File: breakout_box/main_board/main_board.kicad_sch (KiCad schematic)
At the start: 43 parts, among them CN1 19PIN_LEMO, Q1 DMP3099L, Q2 MJD122, Q3 AOZ1360AIL

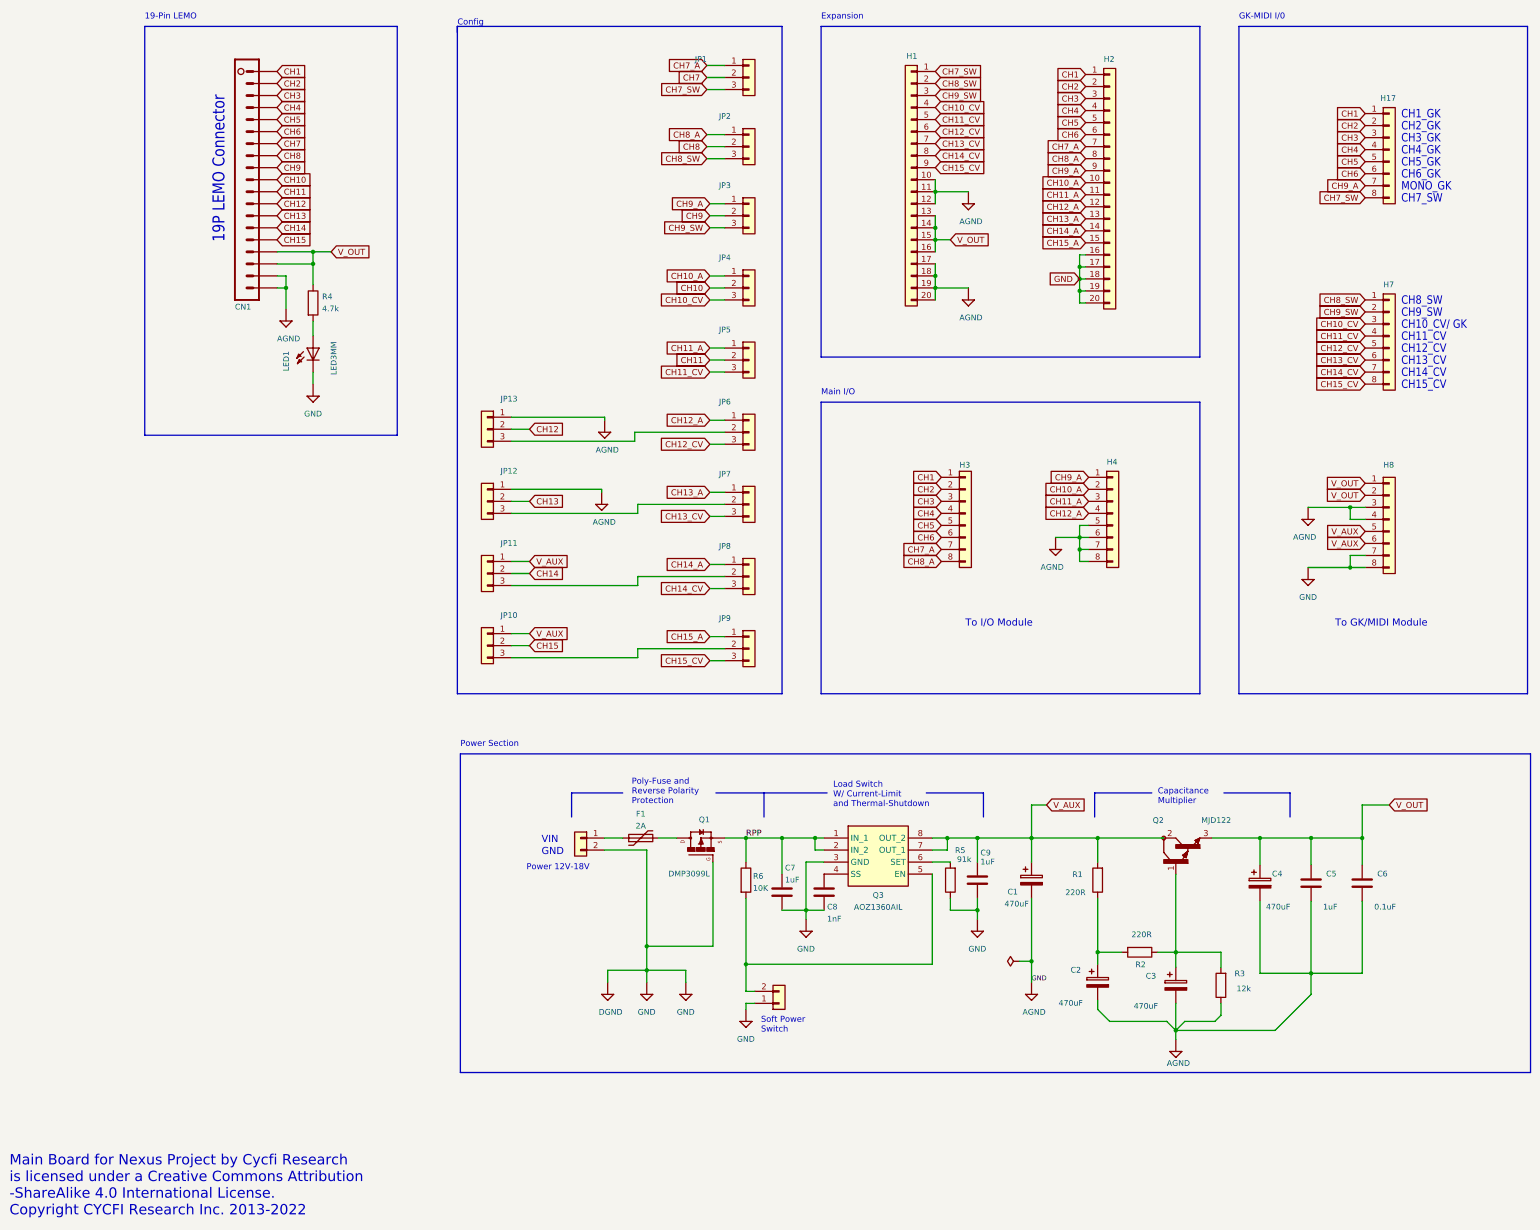
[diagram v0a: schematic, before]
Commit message: Production run May 2025
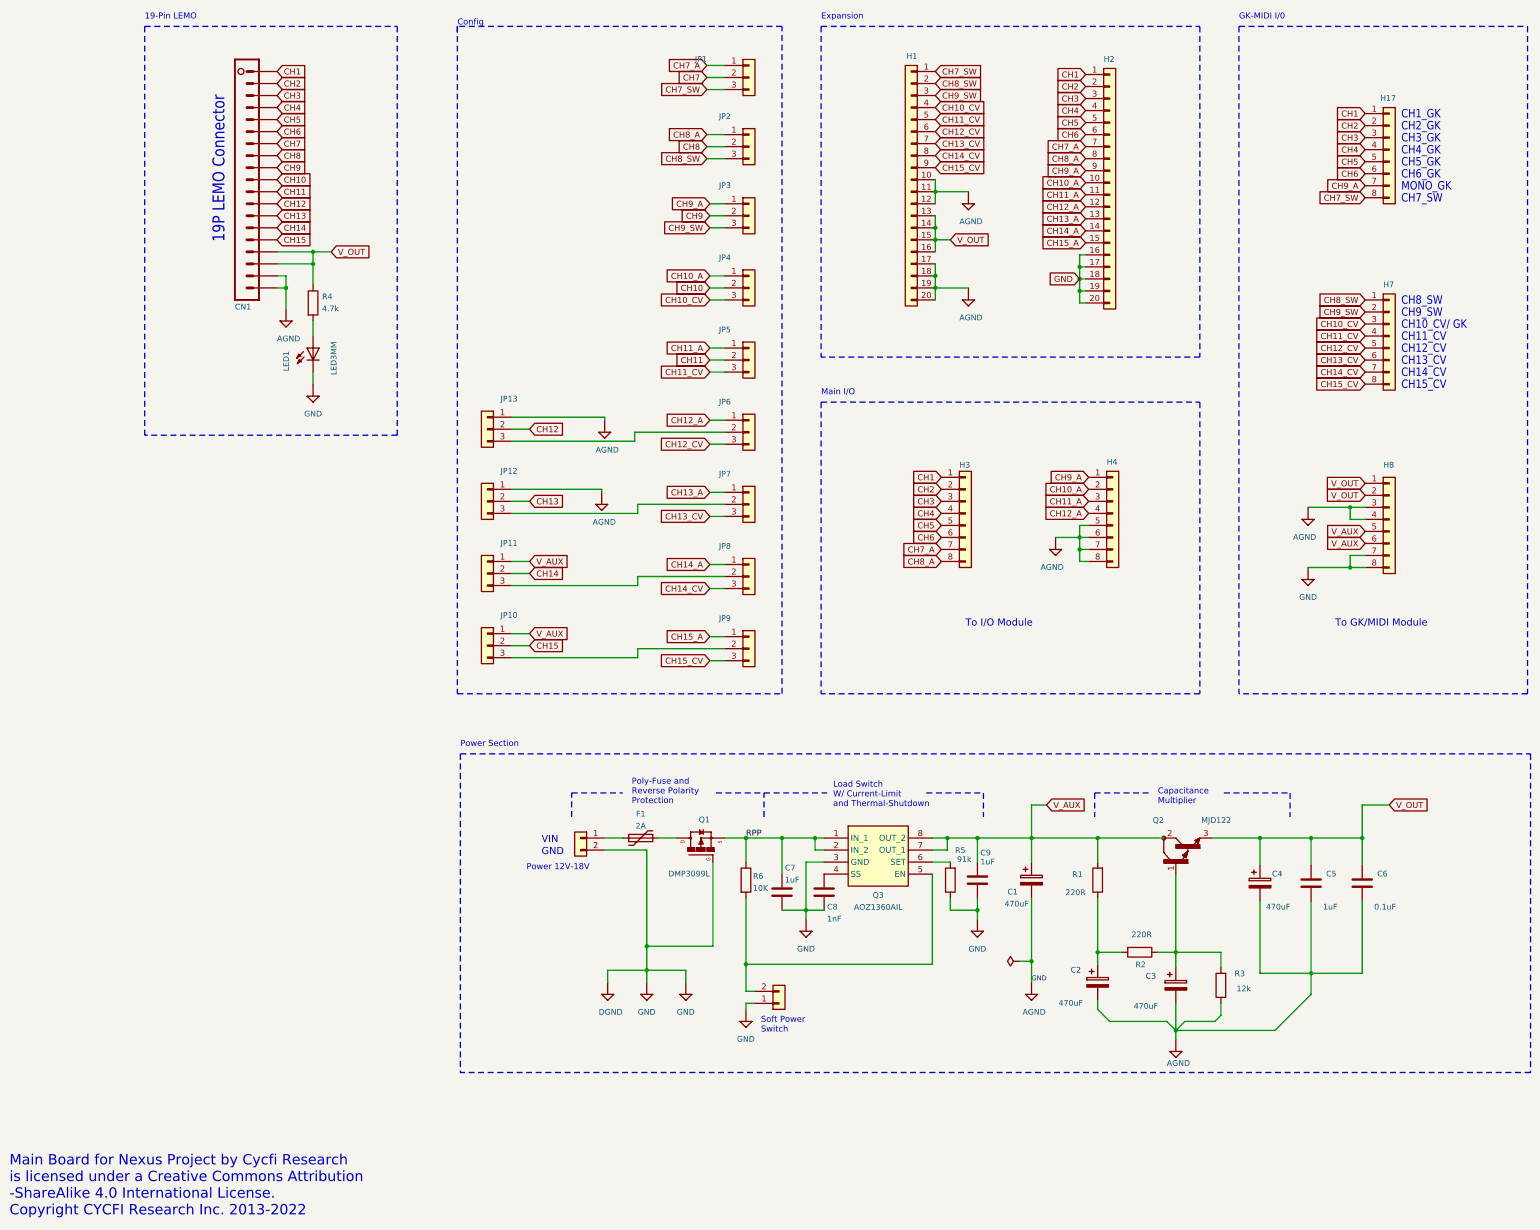
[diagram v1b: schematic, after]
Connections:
- net GND renamed AGND
